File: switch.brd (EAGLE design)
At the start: 11.6 x 31.7 mm, 3 parts

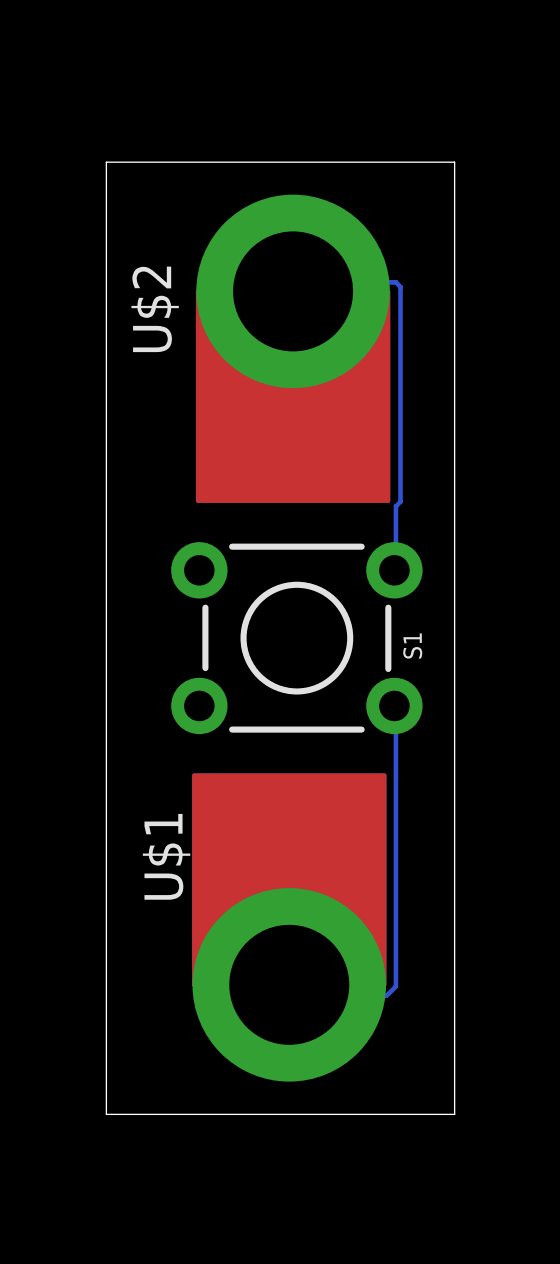
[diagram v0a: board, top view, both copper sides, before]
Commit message: updated
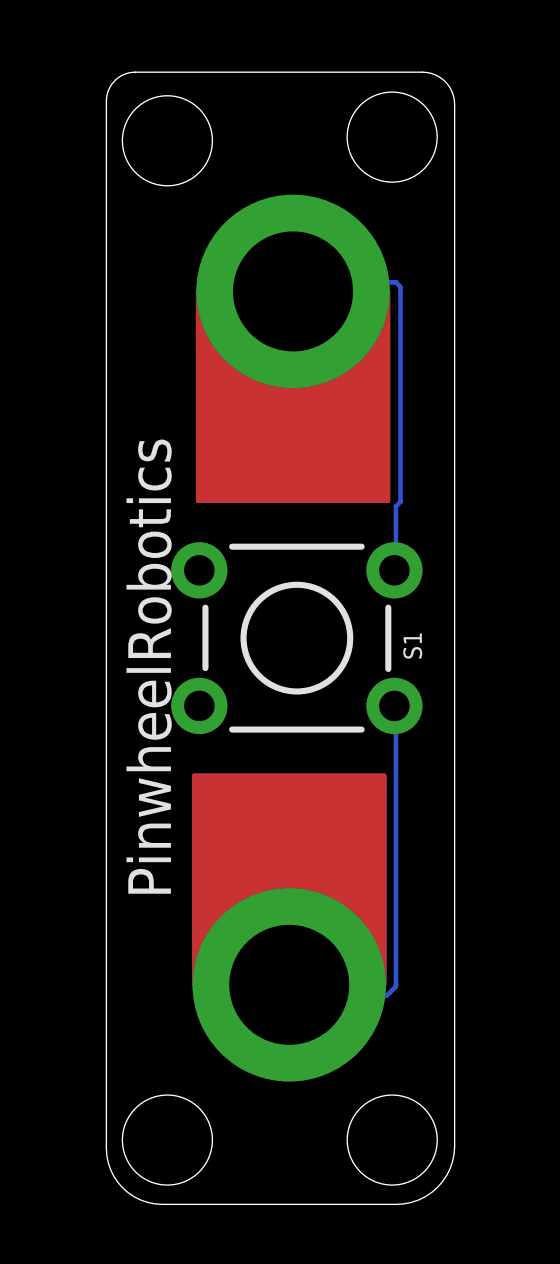
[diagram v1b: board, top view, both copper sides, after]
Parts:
- U$1: value MICROBIT_PAD -> pin1
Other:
- board size 11.6 x 31.7 mm -> 11.6 x 37.7 mm
- board text added: "PinwheelRobotics"
- board text added: "care@pinwheel"
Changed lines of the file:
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@@
 <setting verticaltext="up"/>
 </settings>
-<grid distance="50" unitdist="mil" unit="mm" style="lines" multiple="1" display="yes" altdistance="5" altunitdist="mil" altunit="mm"/>
+<grid distance="0.5" unitdist="mm" unit="mm" style="lines" multiple="1" display="yes" altdistance="5" altunitdist="mil" altunit="mm"/>
 <layers>
 <layer number="1" name="Top" color="4" fill="1" visible="yes" active="yes"/>
@@
 <layer number="43" name="vRestrict" color="2" fill="10" visible="yes" active="yes"/>
 <layer number="44" name="Drills" color="7" fill="1" visible="no" active="yes"/>
-<layer number="45" name="Holes" color="7" fill="1" visible="no" active="yes"/>
+<layer number="45" name="Holes" color="7" fill="1" visible="yes" active="yes"/>
 <layer number="46" name="Milling" color="3" fill="1" visible="no" active="yes"/>
 <layer number="47" name="Measures" color="7" fill="1" visible="no" active="yes"/>
@@
 <board>
 <plain>
-<wire x1="13.97" y1="11.43" x2="25.578" y2="11.43" width="0" layer="20"/>
-<wire x1="25.578" y1="11.43" x2="25.578" y2="43.17" width="0" layer="20"/>
-<wire x1="25.578" y1="43.17" x2="13.97" y2="43.17" width="0" layer="20"/>
-<wire x1="13.97" y1="43.17" x2="13.97" y2="11.43" width="0" layer="20"/>
+<wire x1="13.97" y1="45.206540625" x2="13.97" y2="10.297284375" width="0" layer="20"/>
+<wire x1="13.97" y1="10.297284375" x2="15.837284375" y2="8.43" width="0" layer="20" curve="90"/>
+<wire x1="15.837284375" y1="8.43" x2="23.637571875" y2="8.43" width="0" layer="20"/>
+<wire x1="23.637571875" y1="8.43" x2="25.578" y2="10.370428125" width="0" layer="20" curve="90"/>
+<wire x1="25.578" y1="10.370428125" x2="25.578" y2="45.098121875" width="0" layer="20"/>
+<wire x1="25.578" y1="45.098121875" x2="24.506121875" y2="46.17" width="0" layer="20" curve="90"/>
+<wire x1="24.506121875" y1="46.17" x2="14.933459375" y2="46.17" width="0" layer="20"/>
+<wire x1="14.933459375" y1="46.17" x2="13.97" y2="45.206540625" width="0" layer="20" curve="90"/>
+<hole x="16.004" y="10.574" drill="3"/>
+<hole x="23.498" y="10.574" drill="3"/>
+<hole x="16.004" y="43.884" drill="3"/>
+<hole x="23.496" y="44.006" drill="3"/>
+<text x="16.121" y="18.613" size="1.4224" layer="21" rot="R90">PinwheelRobotics</text>
+<text x="25.35" y="33.449" size="1.4224" layer="22" rot="MR270">care@pinwheel</text>
 </plain>
 <attributes>
@@
 <attribute name="SF_SKU" value="COM-00097" x="-1.27" y="62.865" size="1.778" layer="27" rot="R180" display="off"/>
 </element>
-<element name="U$1" library="microbit" package="MICROBIT_PAD" value="MICROBIT_PAD" x="20.066" y="15.748" smashed="yes" rot="R180">
-<attribute name="NAME" x="15.24" y="21.59" size="1.27" layer="21" rot="R270"/>
-</element>
-<element name="U$2" library="microbit" package="MICROBIT_PAD" value="MICROBIT_PAD" x="20.193" y="38.862" smashed="yes">
-<attribute name="NAME" x="16.129" y="36.703" size="1.27" layer="21" rot="R90"/>
-</element>
+<element name="U$1" library="microbit" package="MICROBIT_PAD" value="pin1" x="20.066" y="15.748" smashed="yes" rot="R180"/>
+<element name="U$2" library="microbit" package="MICROBIT_PAD" value="MICROBIT_PAD" x="20.193" y="38.862" smashed="yes"/>
 </elements>
 <signals>

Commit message: New Updates
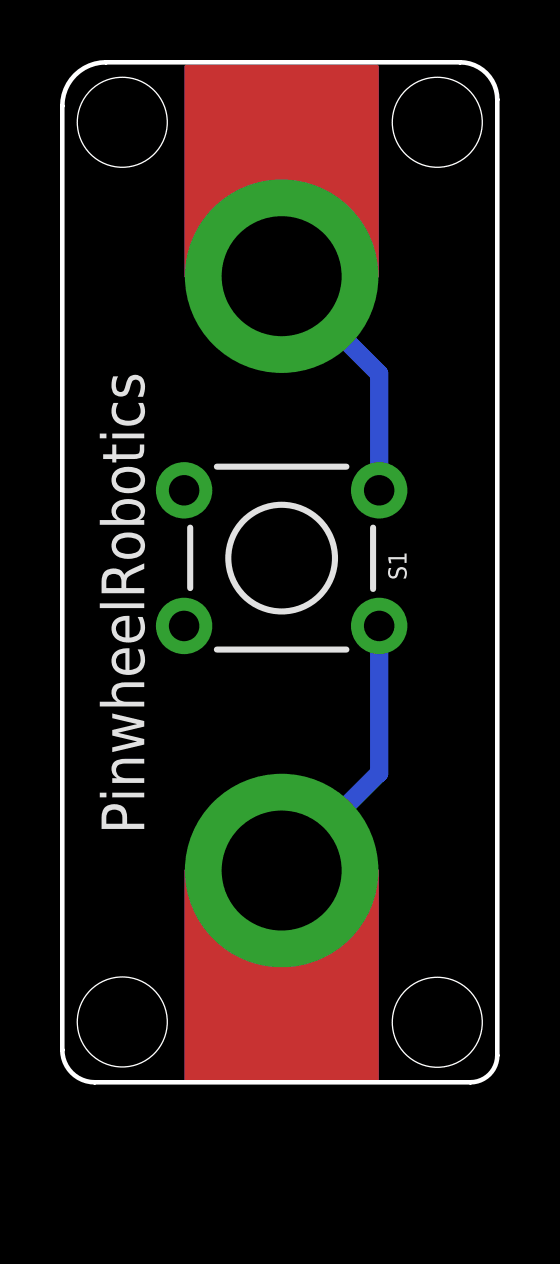
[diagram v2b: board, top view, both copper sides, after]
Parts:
- moved U$1 3.82 mm to (19.8, 19.6), turned to 0 degrees
- moved S1 2.71 mm to (19.8, 30.0)
- moved U$2 0.63 mm to (19.8, 39.4), turned to 180 degrees
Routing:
- net N$2: track 13.3 -> 8.48 mm
- net N$1: track 13.2 -> 9.50 mm
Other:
- board size 11.6 x 37.7 mm -> 14.5 x 34 mm
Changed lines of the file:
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@@
 <drawing>
 <settings>
-<setting alwaysvectorfont="yes"/>
+<setting alwaysvectorfont="no"/>
 <setting verticaltext="up"/>
 </settings>
@@
 <board>
 <plain>
-<wire x1="13.97" y1="45.206540625" x2="13.97" y2="10.297284375" width="0" layer="20"/>
-<wire x1="13.97" y1="10.297284375" x2="15.837284375" y2="8.43" width="0" layer="20" curve="90"/>
-<wire x1="15.837284375" y1="8.43" x2="23.637571875" y2="8.43" width="0" layer="20"/>
-<wire x1="23.637571875" y1="8.43" x2="25.578" y2="10.370428125" width="0" layer="20" curve="90"/>
-<wire x1="25.578" y1="10.370428125" x2="25.578" y2="45.098121875" width="0" layer="20"/>
-<wire x1="25.578" y1="45.098121875" x2="24.506121875" y2="46.17" width="0" layer="20" curve="90"/>
-<wire x1="24.506121875" y1="46.17" x2="14.933459375" y2="46.17" width="0" layer="20"/>
-<wire x1="14.933459375" y1="46.17" x2="13.97" y2="45.206540625" width="0" layer="20" curve="90"/>
-<hole x="16.004" y="10.574" drill="3"/>
-<hole x="23.498" y="10.574" drill="3"/>
-<hole x="16.004" y="43.884" drill="3"/>
-<hole x="23.496" y="44.006" drill="3"/>
-<text x="16.121" y="18.613" size="1.4224" layer="21" rot="R90">PinwheelRobotics</text>
-<text x="25.35" y="33.449" size="1.4224" layer="22" rot="MR270">care@pinwheel</text>
+<hole x="14.5" y="14.511" drill="3"/>
+<hole x="25" y="14.5" drill="3"/>
+<hole x="14.5" y="44.5" drill="3"/>
+<hole x="25" y="44.5" drill="3"/>
+<text x="15.232" y="20.772" size="1.4224" layer="21" rot="R90">PinwheelRobotics</text>
+<text x="26.112" y="34.211" size="1.4224" layer="22" rot="MR270">care@pinwheel</text>
+<wire x1="27" y1="13.394378125" x2="27" y2="45.257834375" width="0.1524" layer="20"/>
+<wire x1="27" y1="45.257834375" x2="25.757834375" y2="46.5" width="0.1524" layer="20" curve="90"/>
+<wire x1="25.757834375" y1="46.5" x2="13.9548875" y2="46.5" width="0.1524" layer="20"/>
+<wire x1="13.9548875" y1="46.5" x2="12.5" y2="45.0451125" width="0.1524" layer="20" curve="90"/>
+<wire x1="12.5" y1="45.0451125" x2="12.5" y2="13.58015" width="0.1524" layer="20"/>
+<wire x1="12.5" y1="13.58015" x2="13.58015" y2="12.5" width="0.1524" layer="20" curve="90"/>
+<wire x1="13.58015" y1="12.5" x2="26.105621875" y2="12.5" width="0.1524" layer="20"/>
+<wire x1="26.105621875" y1="12.5" x2="27" y2="13.394378125" width="0.1524" layer="20" curve="90"/>
 </plain>
 <attributes>
@@
 </autorouter>
 <elements>
-<element name="S1" library="SparkFun-Switches" library_urn="urn:adsk.eagle:library:535" package="TACTILE_SWITCH_PTH_6.0MM" package3d_urn="urn:adsk.eagle:package:40163/1" value="MOMENTARY-SWITCH-SPST-PTH-6.0MM" x="20.32" y="27.305" smashed="yes" rot="R180">
-<attribute name="NAME" x="23.876" y="27.051" size="0.6096" layer="25" font="vector" ratio="20" rot="R270" align="bottom-center"/>
-<attribute name="PROD_ID" value=" SWCH-08441" x="-1.27" y="62.865" size="1.778" layer="27" rot="R180" display="off"/>
-<attribute name="SF_SKU" value="COM-00097" x="-1.27" y="62.865" size="1.778" layer="27" rot="R180" display="off"/>
+<element name="S1" library="SparkFun-Switches" library_urn="urn:adsk.eagle:library:535" package="TACTILE_SWITCH_PTH_6.0MM" package3d_urn="urn:adsk.eagle:package:40163/1" value="MOMENTARY-SWITCH-SPST-PTH-6.0MM" x="19.812" y="29.972" smashed="yes" rot="R180">
+<attribute name="NAME" x="23.368" y="29.718" size="0.6096" layer="25" font="vector" ratio="20" rot="R270" align="bottom-center"/>
+<attribute name="PROD_ID" value=" SWCH-08441" x="-1.778" y="65.532" size="1.778" layer="27" rot="R180" display="off"/>
+<attribute name="SF_SKU" value="COM-00097" x="-1.778" y="65.532" size="1.778" layer="27" rot="R180" display="off"/>
 </element>
-<element name="U$1" library="microbit" package="MICROBIT_PAD" value="pin1" x="20.066" y="15.748" smashed="yes" rot="R180"/>
-<element name="U$2" library="microbit" package="MICROBIT_PAD" value="MICROBIT_PAD" x="20.193" y="38.862" smashed="yes"/>
+<element name="U$1" library="microbit" package="MICROBIT_PAD" value="pin1" x="19.812" y="19.558" smashed="yes"/>
+<element name="U$2" library="microbit" package="MICROBIT_PAD" value="MICROBIT_PAD" x="19.812" y="39.37" smashed="yes" rot="R180"/>
 </elements>
 <signals>
@@
 <contactref element="U$1" pad="PAD"/>
 <contactref element="S1" pad="1"/>
-<wire x1="23.622" y1="15.6972" x2="23.622" y2="24.9936" width="0.1524" layer="16"/>
-<wire x1="23.3172" y1="15.3924" x2="23.622" y2="15.6972" width="0.1524" layer="16"/>
-<wire x1="20.4216" y1="15.3924" x2="23.3172" y2="15.3924" width="0.1524" layer="16"/>
-<wire x1="20.066" y1="15.748" x2="20.4216" y2="15.3924" width="0.1524" layer="16"/>
-<wire x1="23.622" y1="24.9936" x2="23.5712" y2="25.0444" width="0.1524" layer="16"/>
+<wire x1="23.0632" y1="27.7114" x2="23.0632" y2="22.8092" width="0.6096" layer="16"/>
+<wire x1="23.0632" y1="22.8092" x2="19.812" y2="19.558" width="0.6096" layer="16"/>
 </signal>
 <signal name="N$2">
 <contactref element="U$2" pad="PAD"/>
 <contactref element="S1" pad="3"/>
-<wire x1="23.622" y1="31.6992" x2="23.622" y2="29.5656" width="0.1524" layer="16"/>
-<wire x1="23.7744" y1="31.8516" x2="23.622" y2="31.6992" width="0.1524" layer="16"/>
-<wire x1="23.7744" y1="39.0144" x2="23.7744" y2="31.8516" width="0.1524" layer="16"/>
-<wire x1="23.622" y1="39.1668" x2="23.7744" y2="39.0144" width="0.1524" layer="16"/>
-<wire x1="20.574" y1="39.1668" x2="23.622" y2="39.1668" width="0.1524" layer="16"/>
-<wire x1="20.2692" y1="38.862" x2="20.574" y2="39.1668" width="0.1524" layer="16"/>
-<wire x1="23.622" y1="29.5656" x2="23.5712" y2="29.5656" width="0.1524" layer="16"/>
-<wire x1="20.2692" y1="38.862" x2="20.193" y2="38.862" width="0.1524" layer="16"/>
+<wire x1="23.0632" y1="32.2326" x2="23.0632" y2="36.1188" width="0.6096" layer="16"/>
+<wire x1="23.0632" y1="36.1188" x2="19.812" y2="39.37" width="0.6096" layer="16"/>
 </signal>
 </signals>
